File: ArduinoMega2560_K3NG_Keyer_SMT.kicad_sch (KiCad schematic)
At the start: 5 parts, among them J2 Barrel_Jack, J23 Conn_01x02

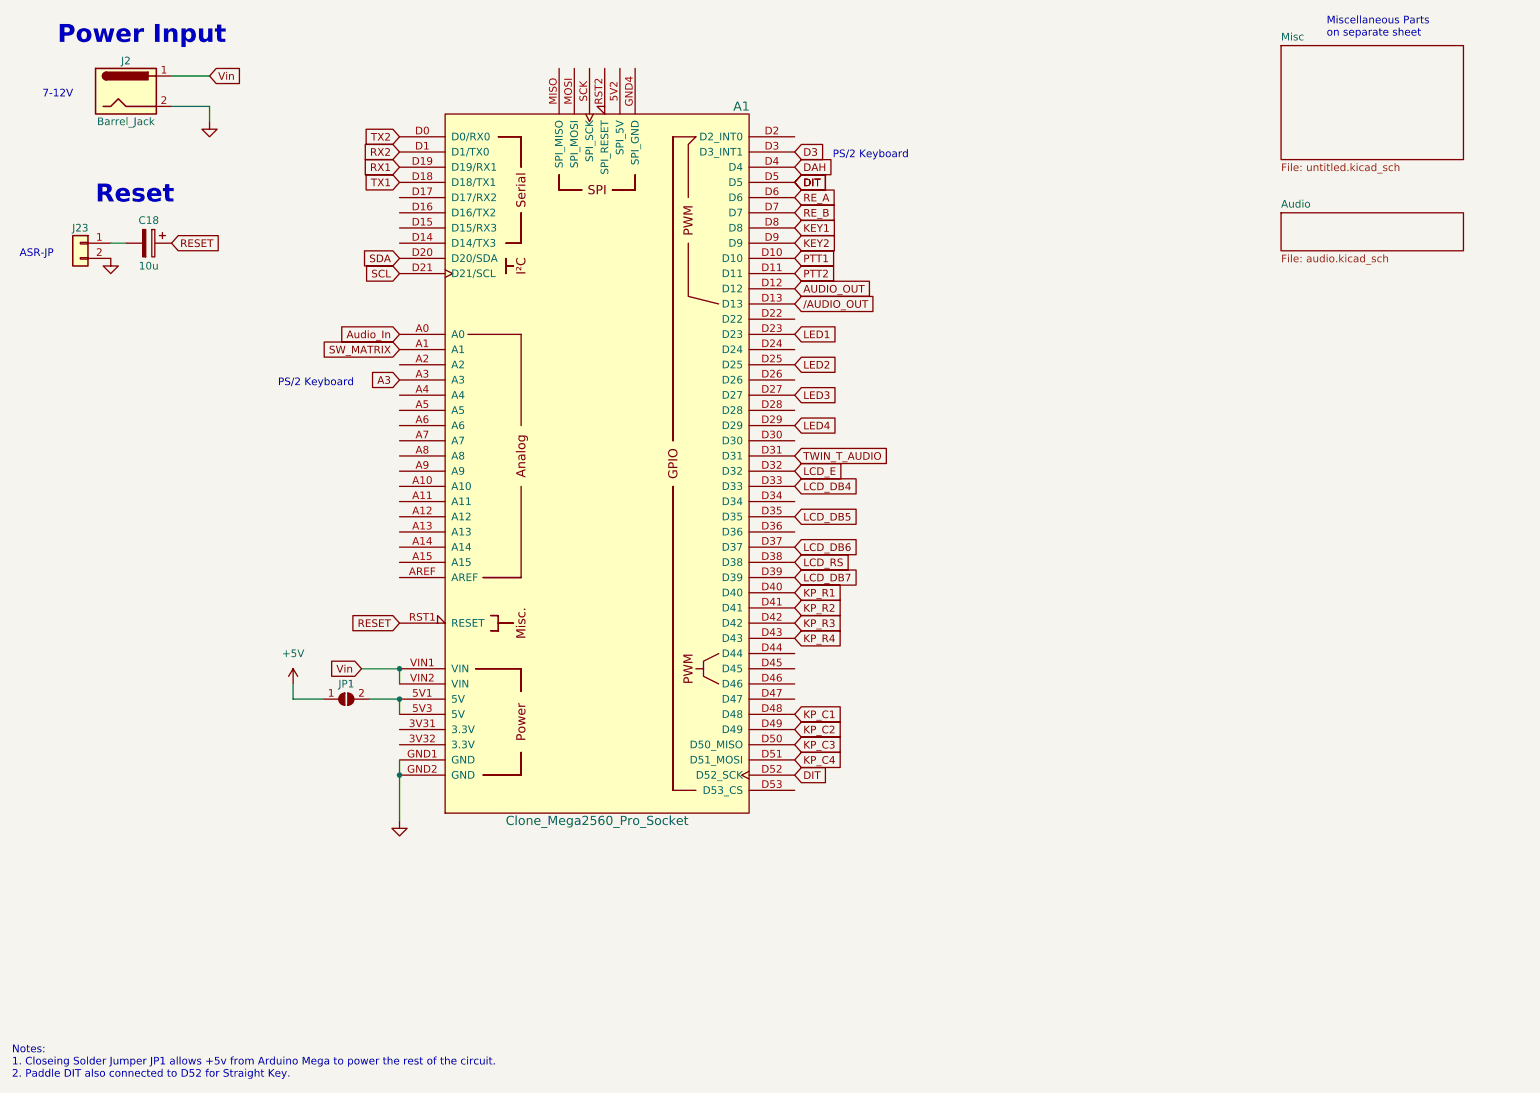
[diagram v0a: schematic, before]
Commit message: Small drawing cleanups.
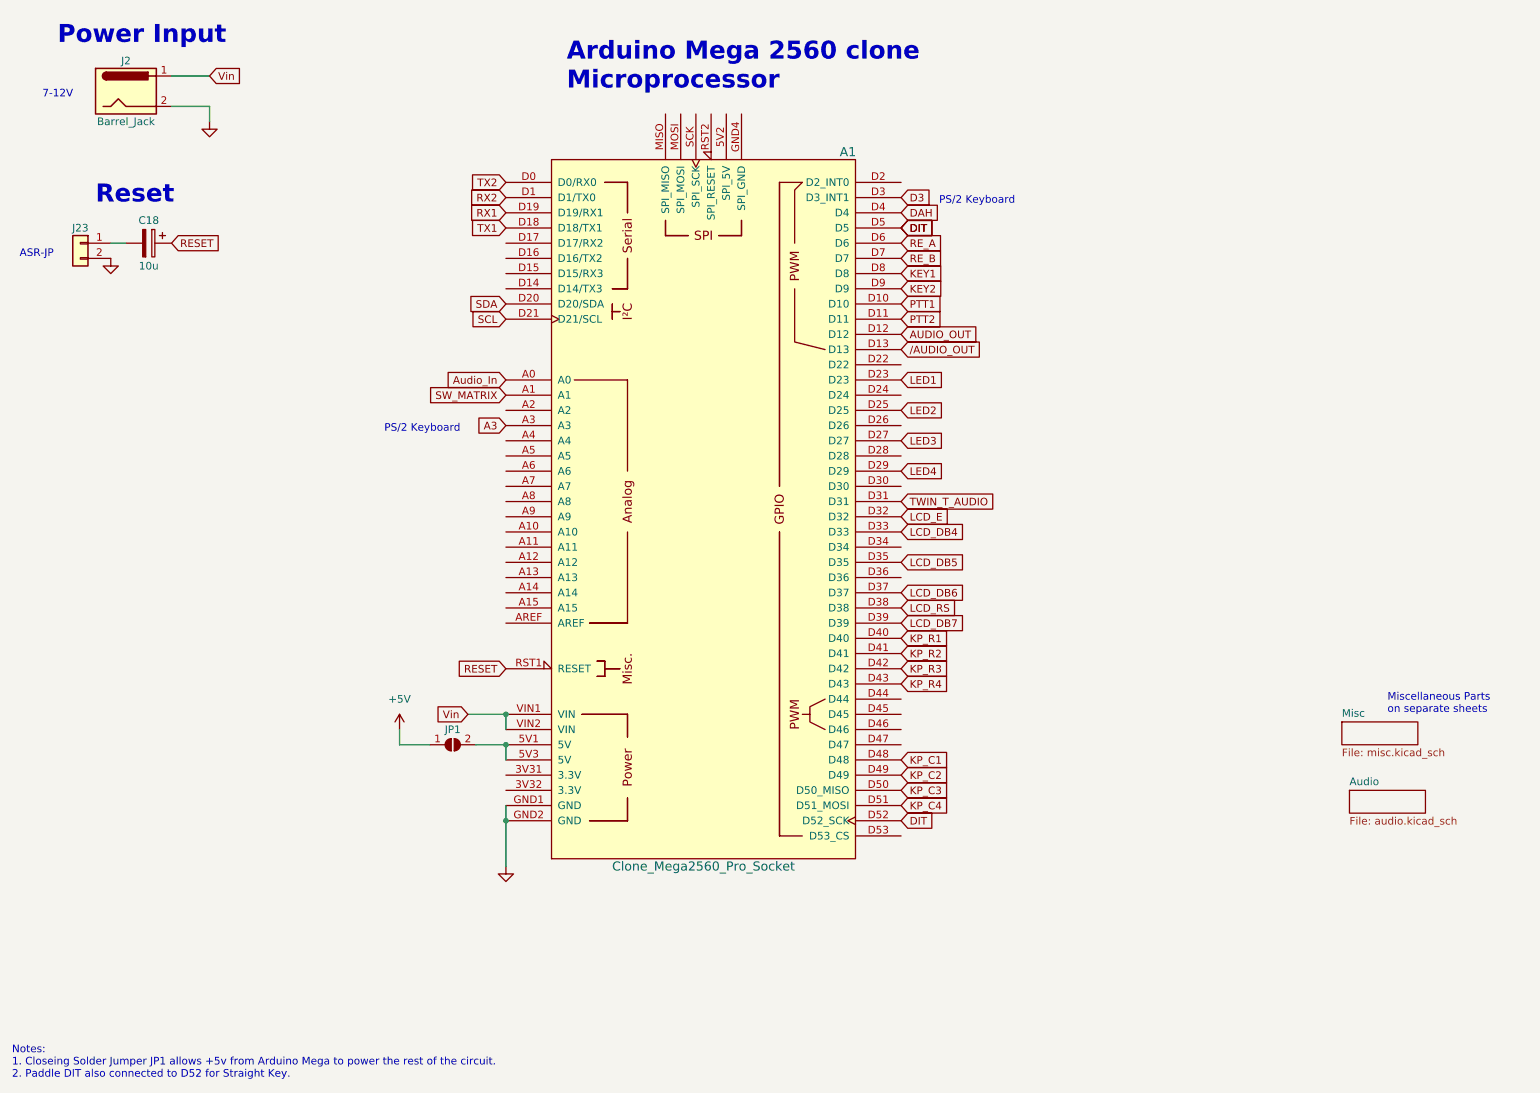
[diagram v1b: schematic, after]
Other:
- sheet Misc: file untitled.kicad_sch -> misc.kicad_sch
- note added: "Arduino Mega 2560 clone Microprocessor"
- note added: "Miscellaneous Parts on separate sheets"
- note removed: "Miscellaneous Parts on separate sheet"
- title: Arduino Mega2560 K3NG Morse Code Keyer - SMT version -> Arduino Mega2560 K3NG Keyer - Microprocessor
- moved on the sheet: A1, JP1
